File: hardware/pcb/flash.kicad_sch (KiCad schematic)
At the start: 0 parts

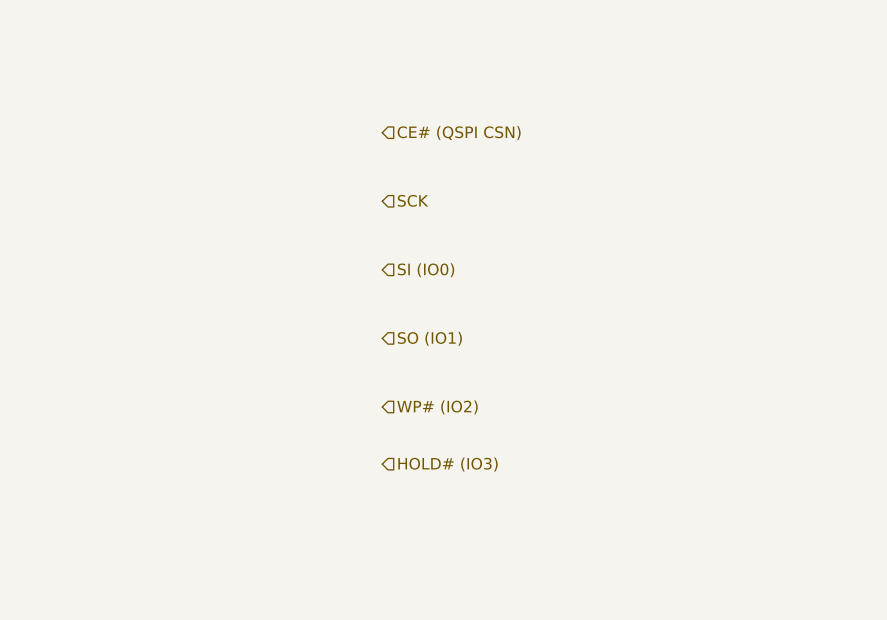
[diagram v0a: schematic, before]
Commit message: Update(hardware): Completed some schematics
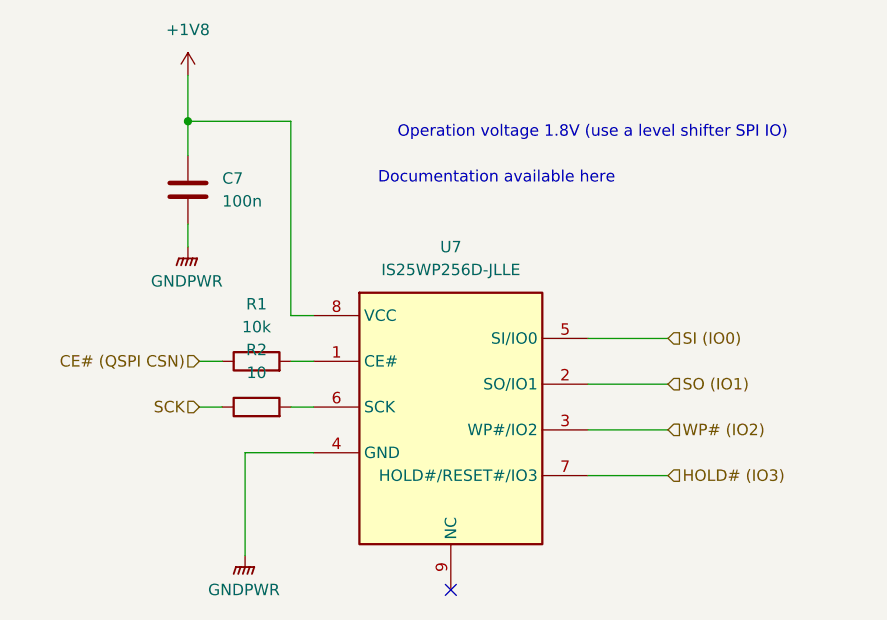
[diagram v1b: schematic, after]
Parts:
- added C7: 100n, Package_SON:WSON-8-1EP_6x5mm_P1.27mm_EP3.4x4.3mm, symbol Device:C
- added R1: 10k, Package_SON:WSON-8-1EP_6x5mm_P1.27mm_EP3.4x4.3mm, symbol Device:R
- added R2: 10, symbol Device:R
- added U7: IS25WP256D-JLLE, Package_SON:WSON-8-1EP_6x5mm_P1.27mm_EP3.4x4.3mm, symbol IS25WP256D-JLLE:IS25WP256D-JLLE
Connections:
- net CE# (QSPI CSN): now also R1.1
- net HOLD# (IO3): now also U7.7 (HOLD#/RESET#/IO3)
- net SCK: now also R2.1
- net SI (IO0): now also U7.5 (SI/IO0)
- net SO (IO1): now also U7.2 (SO/IO1)
- net WP# (IO2): now also U7.3 (WP#/IO2)
- new net: R1.2, U7.1 (CE#)
- new net: R2.2, U7.6 (SCK)
- new net +1V8: C7.1, U7.8 (VCC)
- new net GNDPWR: C7.2, U7.4 (GND)
- no-connect marks 0 -> 1
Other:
- note added: "Documentation available here"
- note added: "Operation voltage 1.8V (use a level shifter SPI IO)"
